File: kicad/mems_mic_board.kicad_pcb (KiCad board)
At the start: 2 copper layers, 10 parts, among them J1 Conn_01x02_Male, J2 Conn_01x03_Male, J3 Conn_01x06_Male, J4 Conn_01x02_Male, J5 Conn_01x04_Male, J6 Conn_01x08_Male, J7 Conn_01x08_Male, U1 tactile_sw, U2 mems_mic, U3 mems_mic

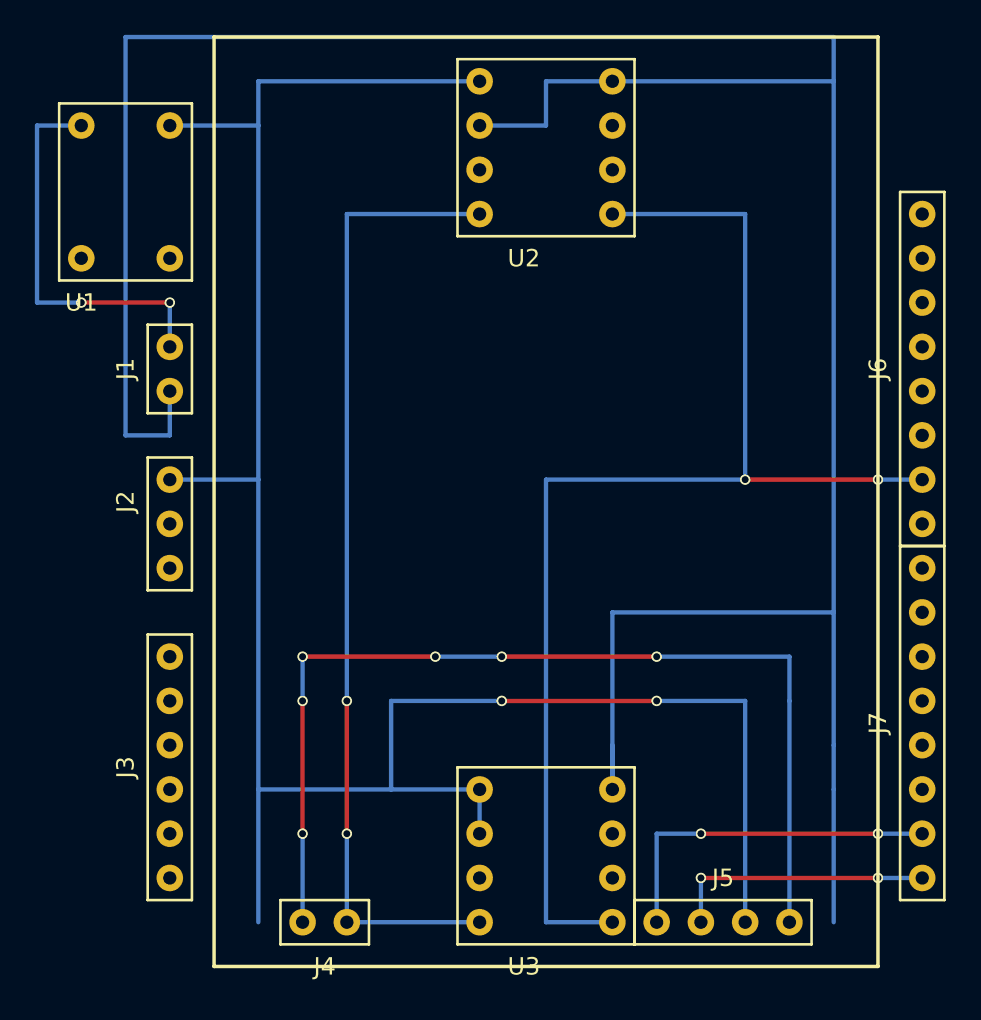
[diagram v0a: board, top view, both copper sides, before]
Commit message: update
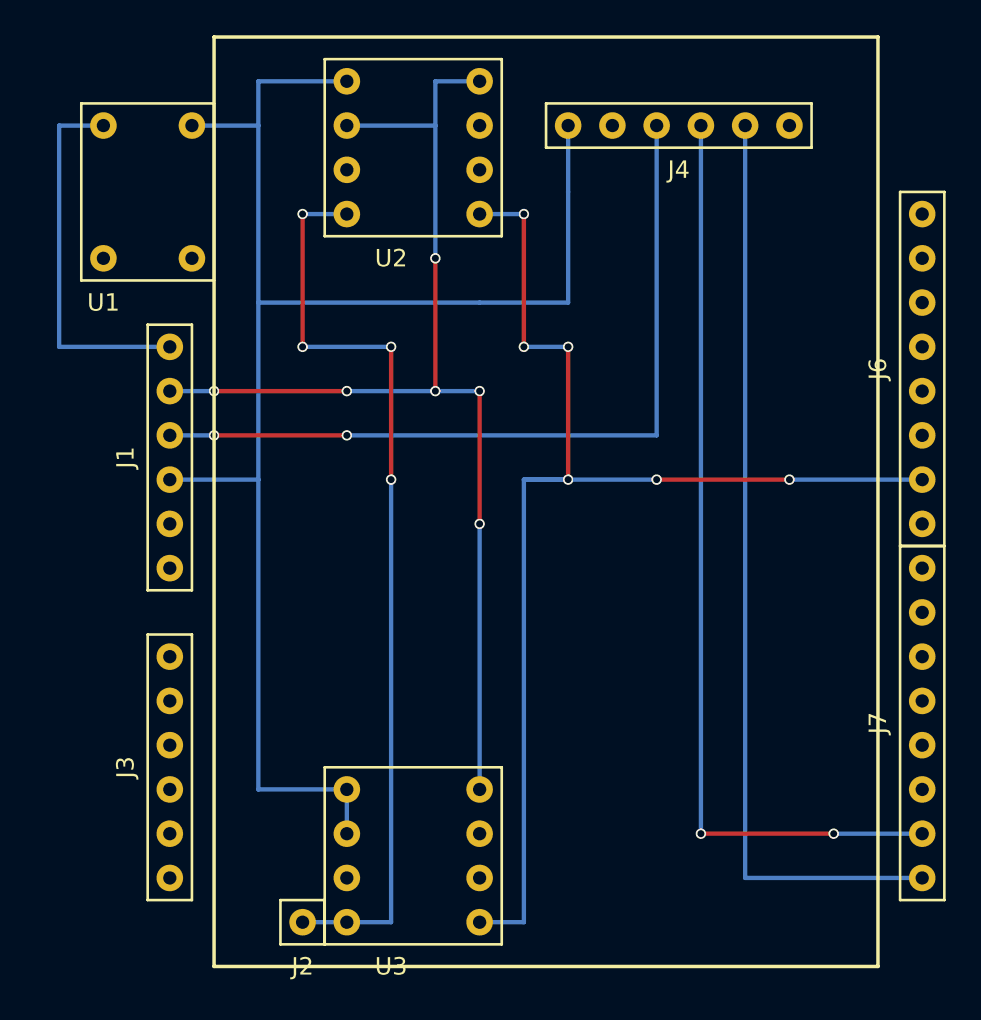
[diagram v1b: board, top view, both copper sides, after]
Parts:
- removed J5: Conn_01x04_Male, mcu:Pin Header 4P
- J1: value Conn_01x02_Male -> Conn_01x06_Male; footprint mcu:Pin Header 2P -> mcu:Pin Header 6P
- J2: value Conn_01x03_Male -> Conn_01x01_Male; footprint mcu:Pin_Header_3P -> mcu:Pin_header_1P
- J4: value Conn_01x02_Male -> Conn_01x06_Female; footprint mcu:Pin Header 2P -> mcu:Pin Header 6P
- moved J4 50.0 mm to (141.0, 90.2)
- moved J2 24.1 mm to (119.4, 135.9), turned to 0 degrees
- moved U2 7.62 mm to (125.7, 91.4)
- moved U3 7.62 mm to (125.7, 132.1)
- moved J1 5.08 mm to (111.8, 109.2)
- moved U1 1.27 mm to (110.5, 94.0)
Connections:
- J2 pad 1: GND -> Net-(J2-Pad1)
- J4 pad 1: Net-(J4-Pad1) -> GND
- J7 pad 7: Net-(J5-Pad4) -> Net-(J4-Pad4)
- J7 pad 8: Net-(J5-Pad3) -> Net-(J4-Pad5)
- U2 pad 4: Net-(J4-Pad2) -> Net-(J2-Pad1)
- U3 pad 4: Net-(J4-Pad2) -> Net-(J2-Pad1)
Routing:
- net +3V3: track 167.6 -> 66.0 mm, vias 0 -> 6
- net Net-(J4-Pad1): track 58.4 -> 0.00 mm, vias 6 -> 0
- net Net-(J4-Pad2): track 55.9 -> 0.00 mm, vias 2 -> 0
- net Net-(J4-Pad5): track 0.00 -> 53.3 mm
- net Net-(J4-Pad4): track 0.00 -> 53.3 mm, vias 0 -> 2
- net Net-(J2-Pad1): track 0.00 -> 53.3 mm, vias 0 -> 4
- net Net-(J1-Pad3): track 0.00 -> 45.7 mm, vias 0 -> 2
- net GND: track 124.5 -> 90.2 mm, vias 2 -> 0
- net Net-(J5-Pad4): track 20.3 -> 0.00 mm, vias 2 -> 0
- net Net-(J5-Pad3): track 15.2 -> 0.00 mm, vias 2 -> 0
- net Net-(J1-Pad1): track 22.9 -> 21.6 mm, vias 2 -> 0
- net Net-(J6-Pad7): vias 2 -> 6
